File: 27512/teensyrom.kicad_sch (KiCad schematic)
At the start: 4 parts, among them J1 Conn_01x07_Pin, U1 27512, U2 2716, U3 Teensy 4.1 module

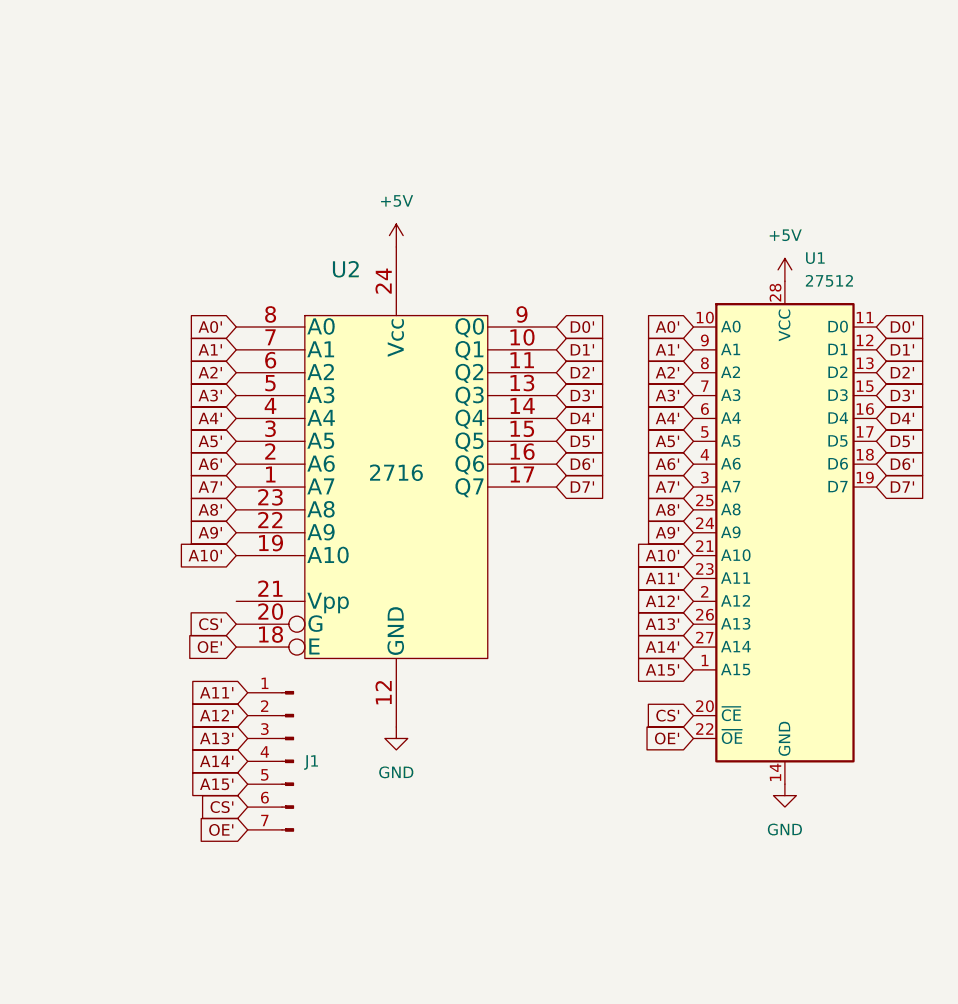
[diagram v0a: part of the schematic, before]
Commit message: update schematic pdfs
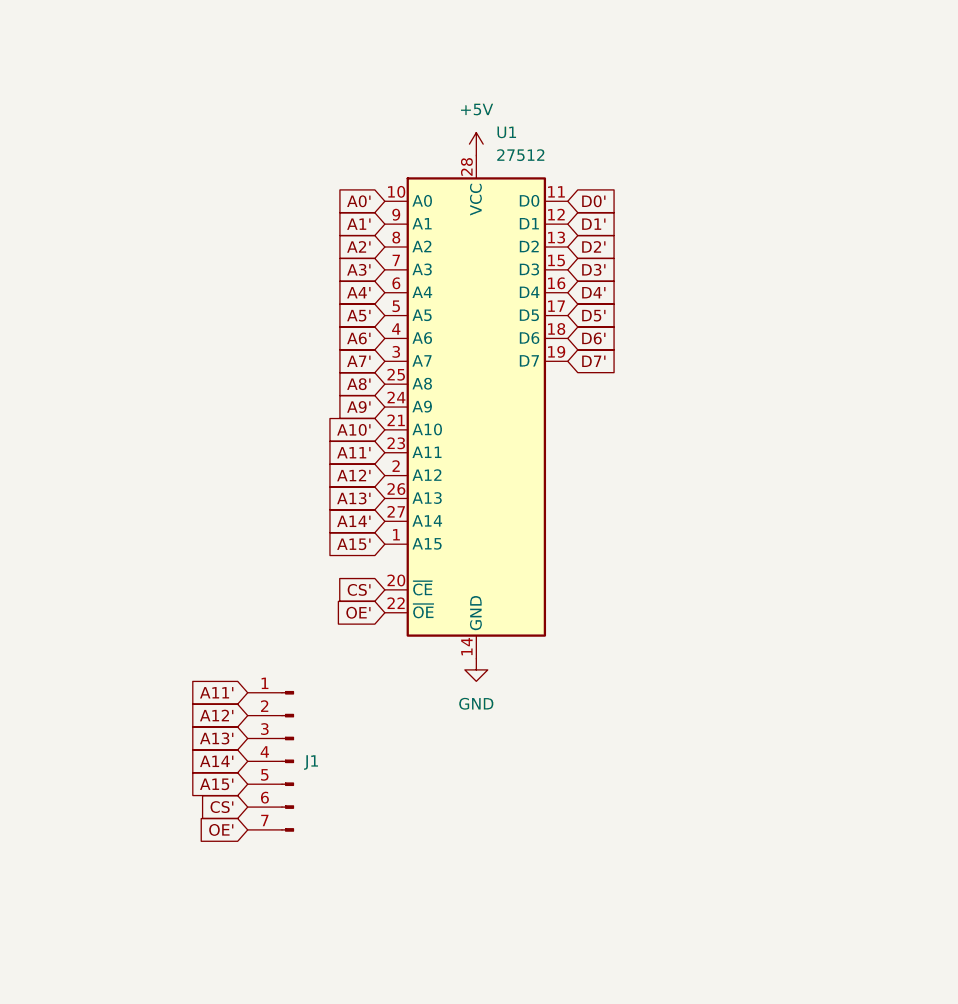
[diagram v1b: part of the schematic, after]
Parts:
- removed U2: 2716, Package_DIP:DIP-24_W15.24mm, symbol memory:2716
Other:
- moved on the sheet: U1
